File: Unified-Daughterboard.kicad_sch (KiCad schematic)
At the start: 9 parts, among them J1 HRO-TYPE-C-31-M-12, J2 Conn_01x04

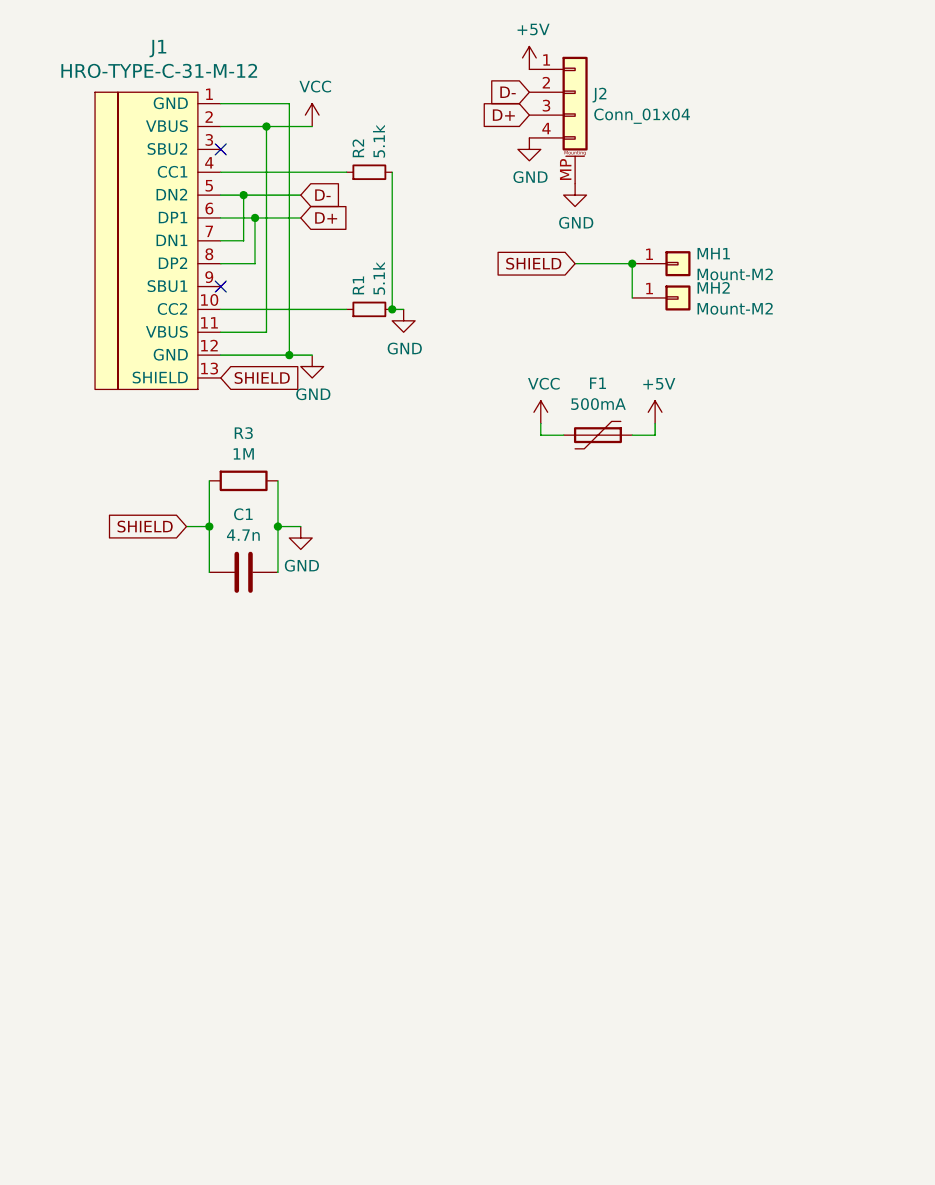
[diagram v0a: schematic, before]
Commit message: update dboard
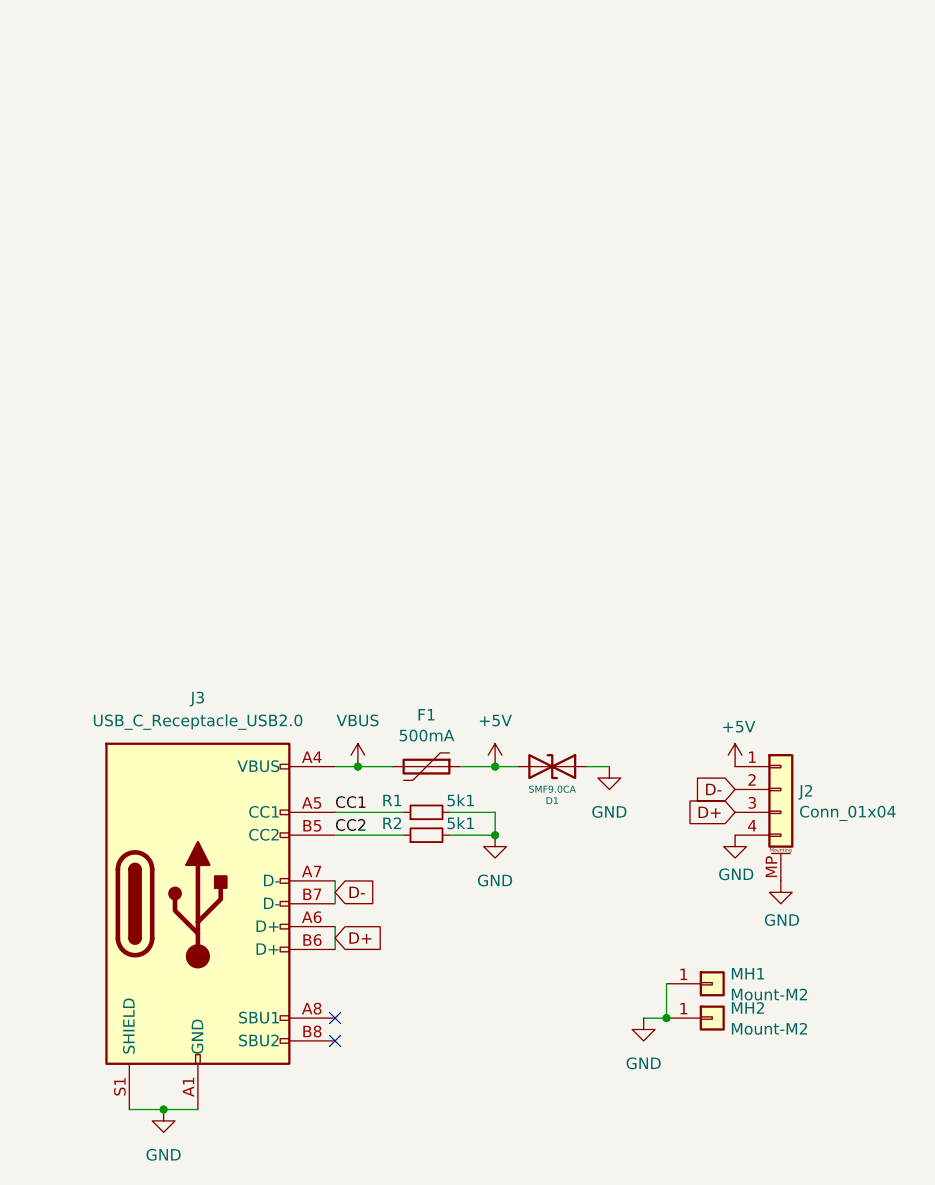
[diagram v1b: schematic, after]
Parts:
- removed C1: 4.7n, Capacitor_SMD:C_0603_1608Metric, symbol Device:C
- removed J1: HRO-TYPE-C-31-M-12, Type-C:HRO-TYPE-C-31-M-12-jlc, symbol Type-C:HRO-TYPE-C-31-M-12
- removed R3: 1M, Resistor_SMD:R_0805_2012Metric, symbol Device:R
- added D1: SMF9.0CA, Diode_SMD:D_SOD-123, symbol Device:D_TVS
- added J3: USB_C_Receptacle_USB2.0, Connector_USB:USB_C_Receptacle_HRO_TYPE-C-31-M-12, symbol Connector:USB_C_Receptacle_USB2.0
- R1, R2: value 5.1k -> 5k1; footprint Resistor_SMD:R_0603_1608Metric -> Resistor_SMD:R_0402_1005Metric; LCSC C23186 -> (none)
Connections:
- net SHIELD is gone; now on net GND: MH1.1 (Pin_1), MH2.1 (Pin_1)
- net +5V: now also D1.2 (A2)
- net D+: now also J3.A6 (D+), J3.B6 (D+)
- net D-: now also J3.A7 (D-), J3.B7 (D-)
- net GND: now also D1.1 (A1), J3.A1 (GND), J3.A12 (GND), J3.B1 (GND), J3.B12 (GND), J3.S1 (SHIELD)
- net CC1: now reaches R1.1
- net CC1: now also J3.A5 (CC1)
- net CC2: now reaches R2.1
- net CC2: now also J3.B5 (CC2)
- net VCC renamed VBUS
- net VBUS: now also J3.A4 (VBUS), J3.A9 (VBUS), J3.B4 (VBUS), J3.B9 (VBUS)
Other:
- moved on the sheet: F1, J2, MH1, MH2
